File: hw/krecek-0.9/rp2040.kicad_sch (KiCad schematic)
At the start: 10 parts, among them U1 RP2040, U2 W25Q128JVS, U4 XL9555, X1 X322512MSB4SI

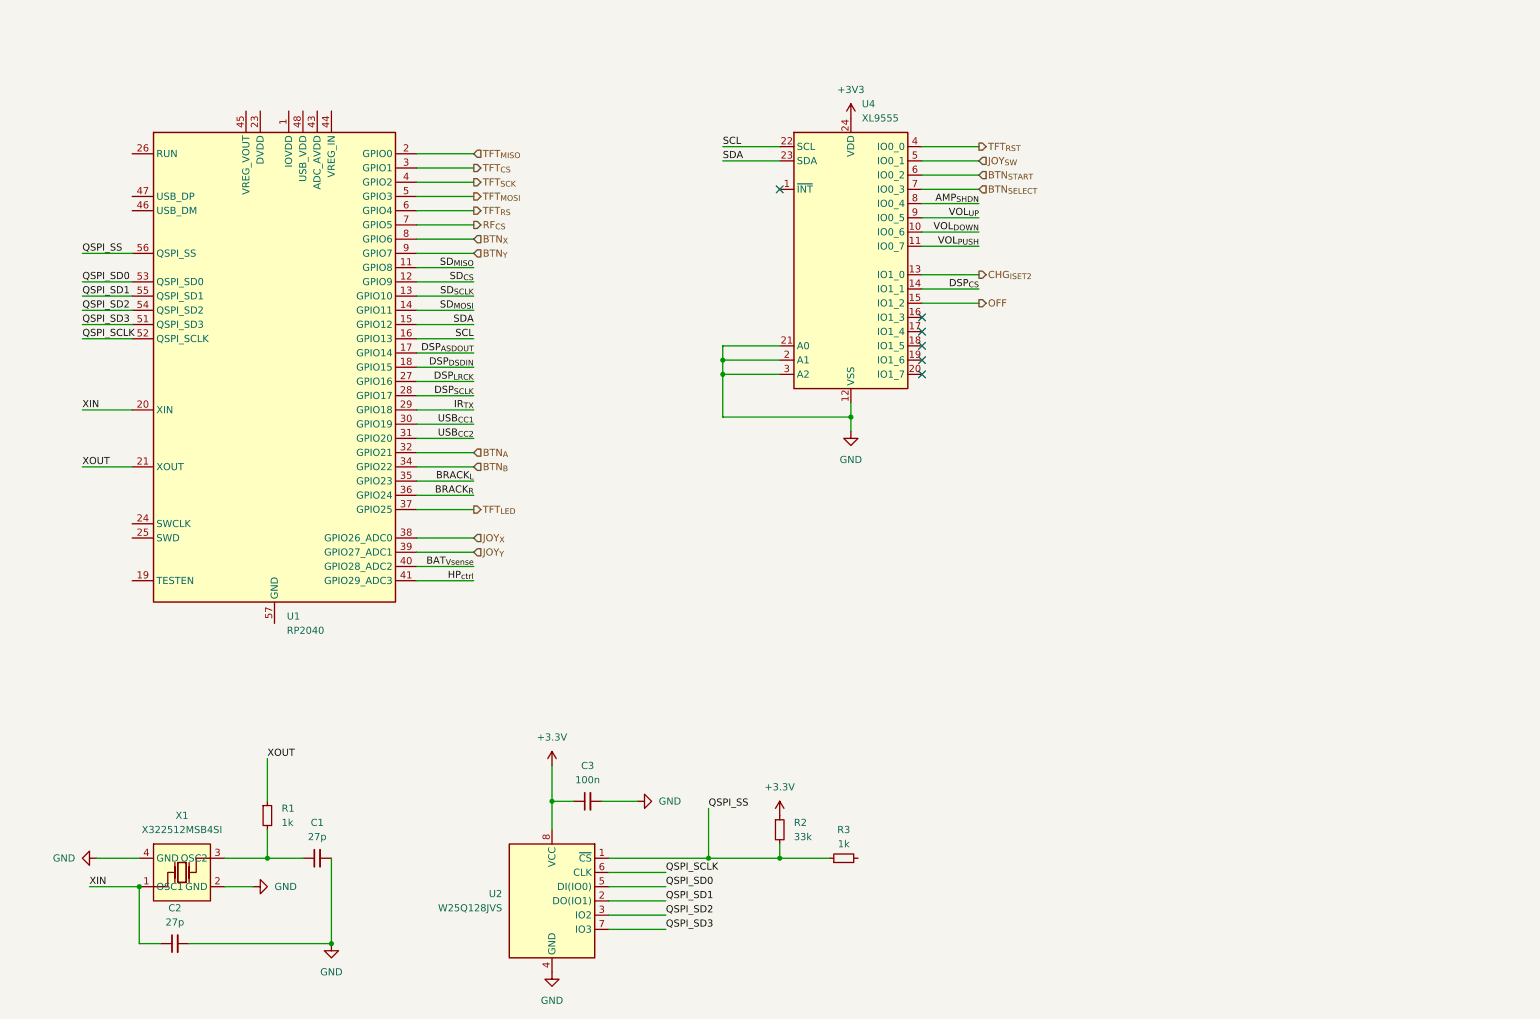
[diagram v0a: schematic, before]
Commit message: Update schematic
Signed-off-by: Jan Hamal Dvořák <mordae@anilinux.org>
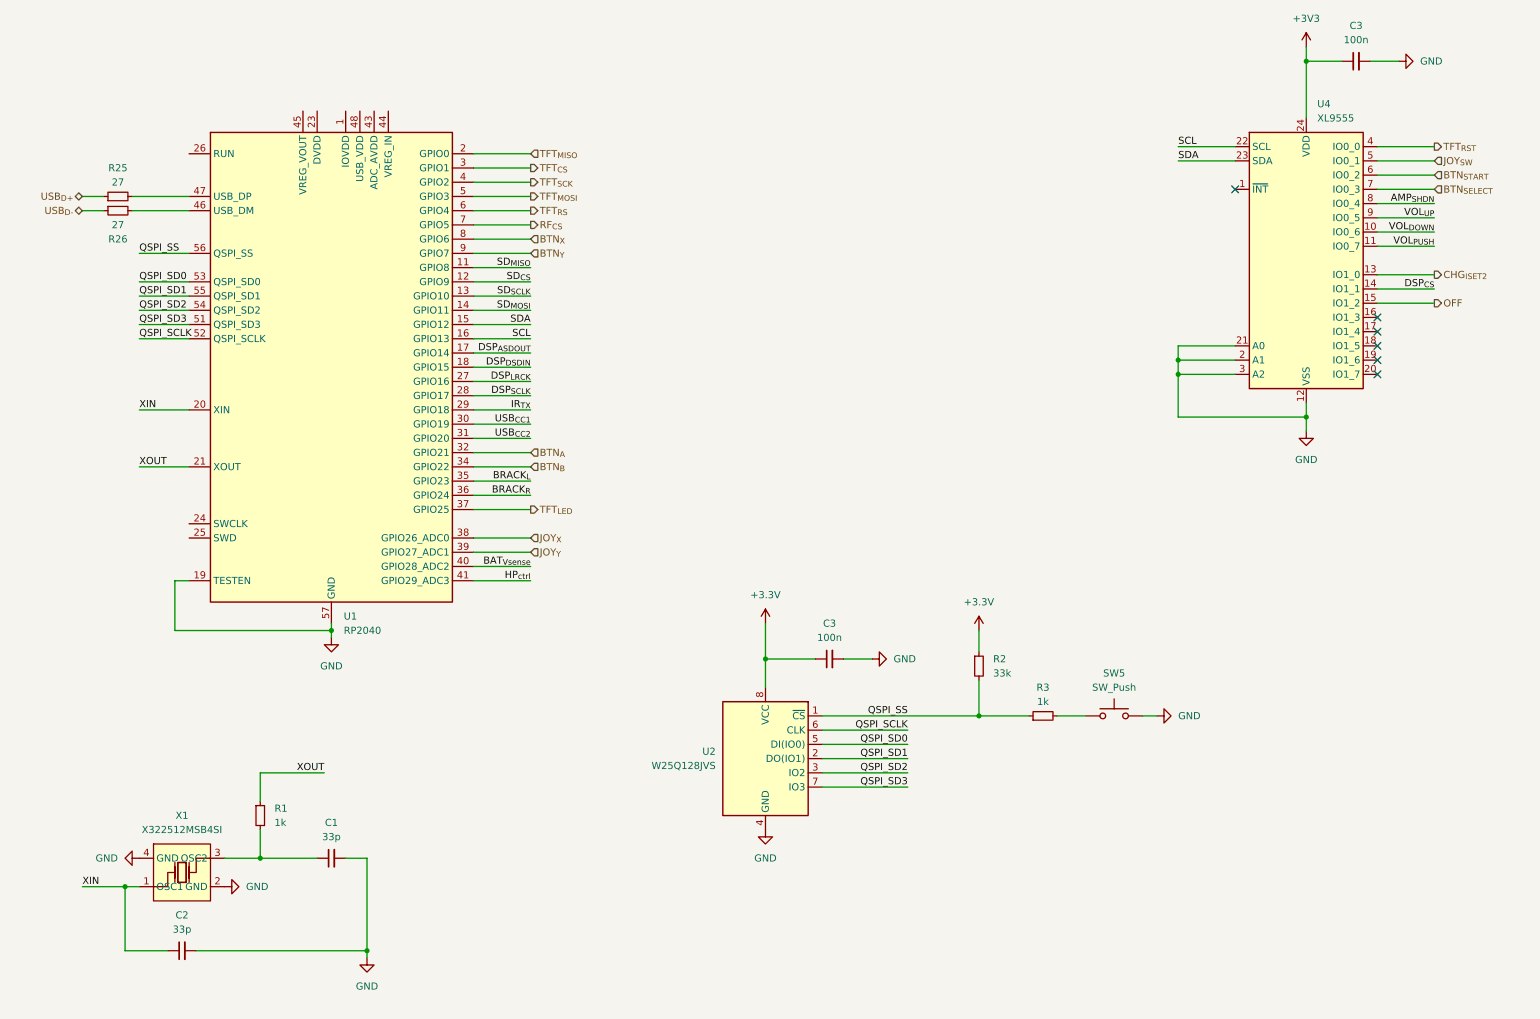
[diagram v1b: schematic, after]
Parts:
- added C3: 100n, Capacitor_SMD:C_0402_1005Metric, symbol Device:C_Small
- added R25, R26: 27, Resistor_SMD:R_0603_1608Metric, symbol Device:R_Small
- added SW5: SW_Push, LCSC:SW-SMD_4P-L5.1-W5.1-P3.70-LS6.5-TL-2, symbol Switch:SW_Push
- C1, C2: value 27p -> 33p; footprint (none) -> Capacitor_SMD:C_0402_1005Metric; LCSC Part (none) -> C1562
- C3: footprint (none) -> Capacitor_SMD:C_0402_1005Metric; LCSC Part (none) -> C307331
- R1, R3: footprint (none) -> Resistor_SMD:R_0402_1005Metric; LCSC Part (none) -> C11702
- R2: footprint (none) -> Capacitor_SMD:C_0402_1005Metric; LCSC Part (none) -> C25779
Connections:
- net +3V3: now also C3.1
- net GND: now also U1.19 (TESTEN), U1.57 (GND), C3.2, SW5.2
- net at R3.2: now also SW5.1
- net at U1.46 (USB_DM): now also R26.2
- net at U1.47 (USB_DP): now also R25.2
- new net USB_{D+}: R25.1
- new net USB_{D-}: R26.1
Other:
- moved on the sheet: C1, C2, C3, R1, R2, R3, U1, U2, U4

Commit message: Further tweaks and improvements
- Use a nicer schematic template
- Tie START button with power on
- Add ferrite to USB shield
- Add CC1/CC2 makeshift ADC
- Tidy up schematics a little bit

Signed-off-by: Jan Hamal Dvořák <mordae@anilinux.org>
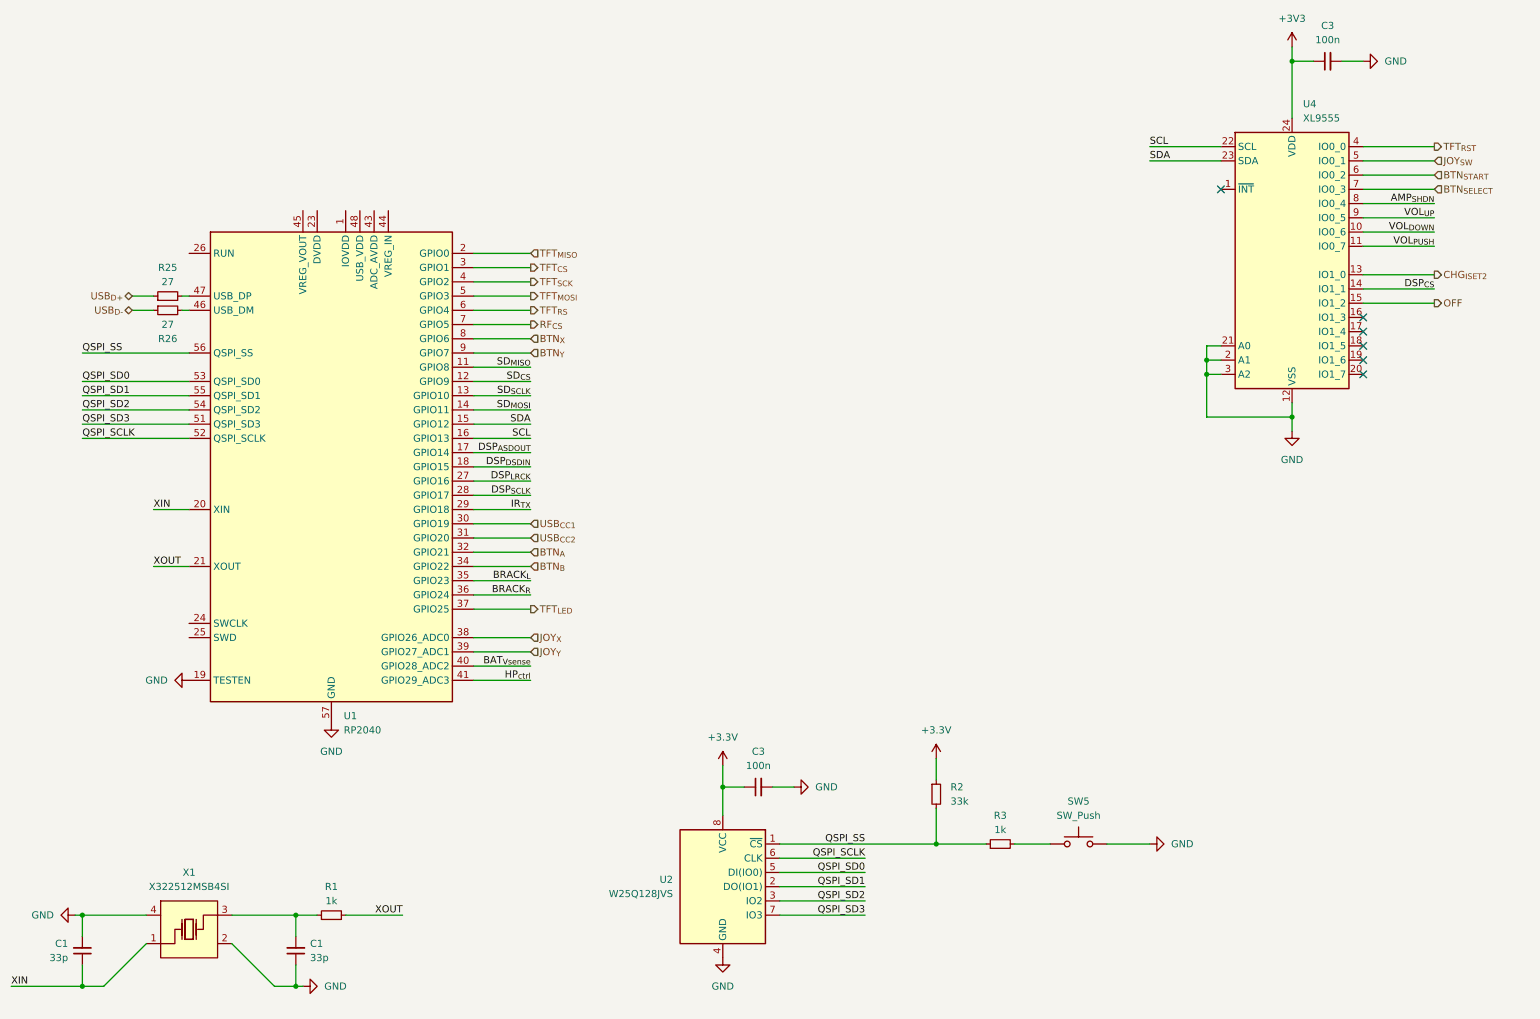
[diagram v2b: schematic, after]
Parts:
- removed C2: 33p, Capacitor_SMD:C_0402_1005Metric, symbol Device:C_Small
- added C1: 33p, Capacitor_SMD:C_0402_1005Metric, symbol Device:C_Small
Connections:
- net GND: now also C1.1, C1.2; no longer C1.2
- net XIN: now also C1.1
- net XOUT: now also R1.2; no longer R1.1
- new net: C1.2, R1.1, X1.3 (OSC2)
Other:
- company: (none) -> DDM Spirála
- title: (none) -> Křeček
- moved on the sheet: C1, C3, R1, R2, R25, R26, R3, SW5, U1, U2, U4
